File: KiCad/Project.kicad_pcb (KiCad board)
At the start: 2 copper layers, 138.4 x 74.9 mm, 73 parts, among them IC1 ATMEGA328-P, IC2 ATTINY85-P, IC3 ATTINY85-P, M1 Motor, M2 Motor, P1 CONN_02X03, P2 CONN_01X02, P3 CONN_01X02, P4 CONN_01X02, P5 CONN_02X04, P6 CONN_02X03, P7 CONN_01X02, Q1 Q_NPN_BCE, Q2 Q_NPN_BCE, Q4 Q_NPN_BCE, Q5 NPN, SW4 SW_PUSH, U1 BlueSmirf, U2 LM317, U3 LM317, U6 SN754410NE, Y1 Crystal

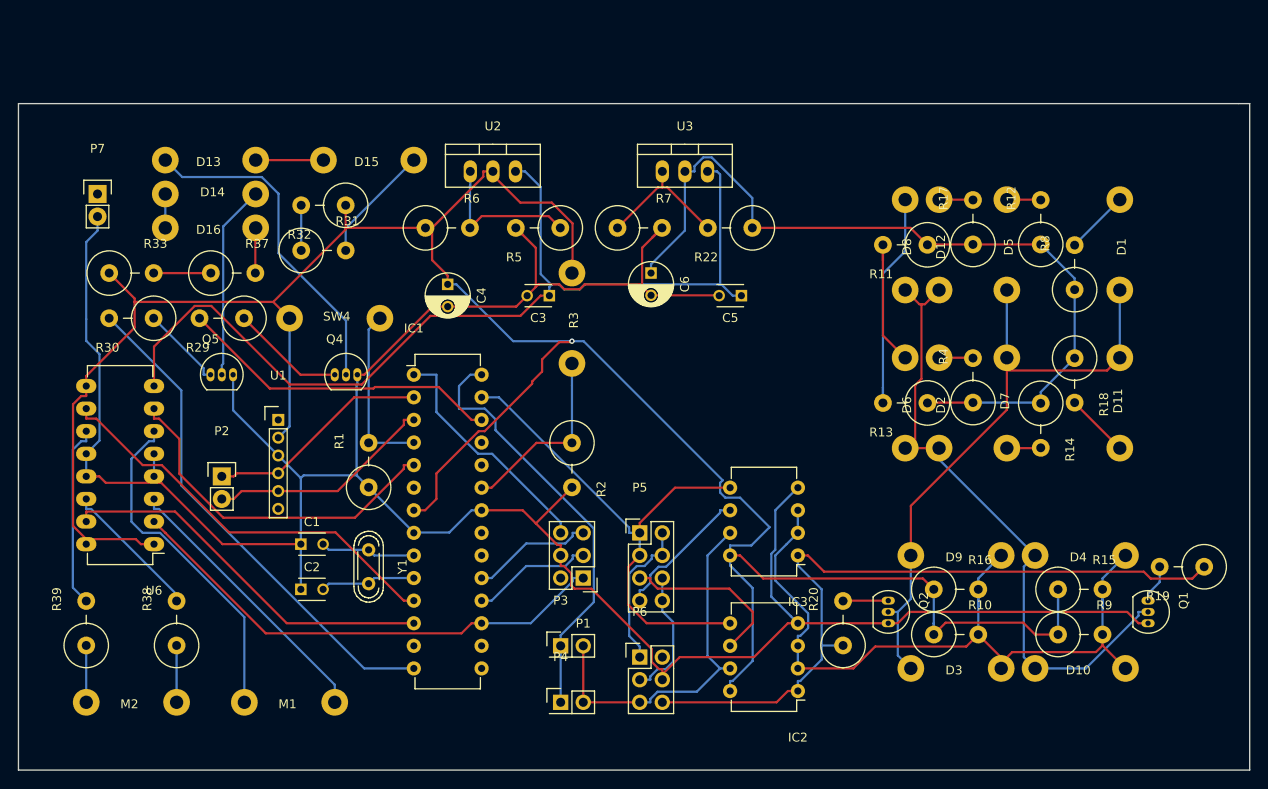
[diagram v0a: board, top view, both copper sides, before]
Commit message: Added smaller footprints
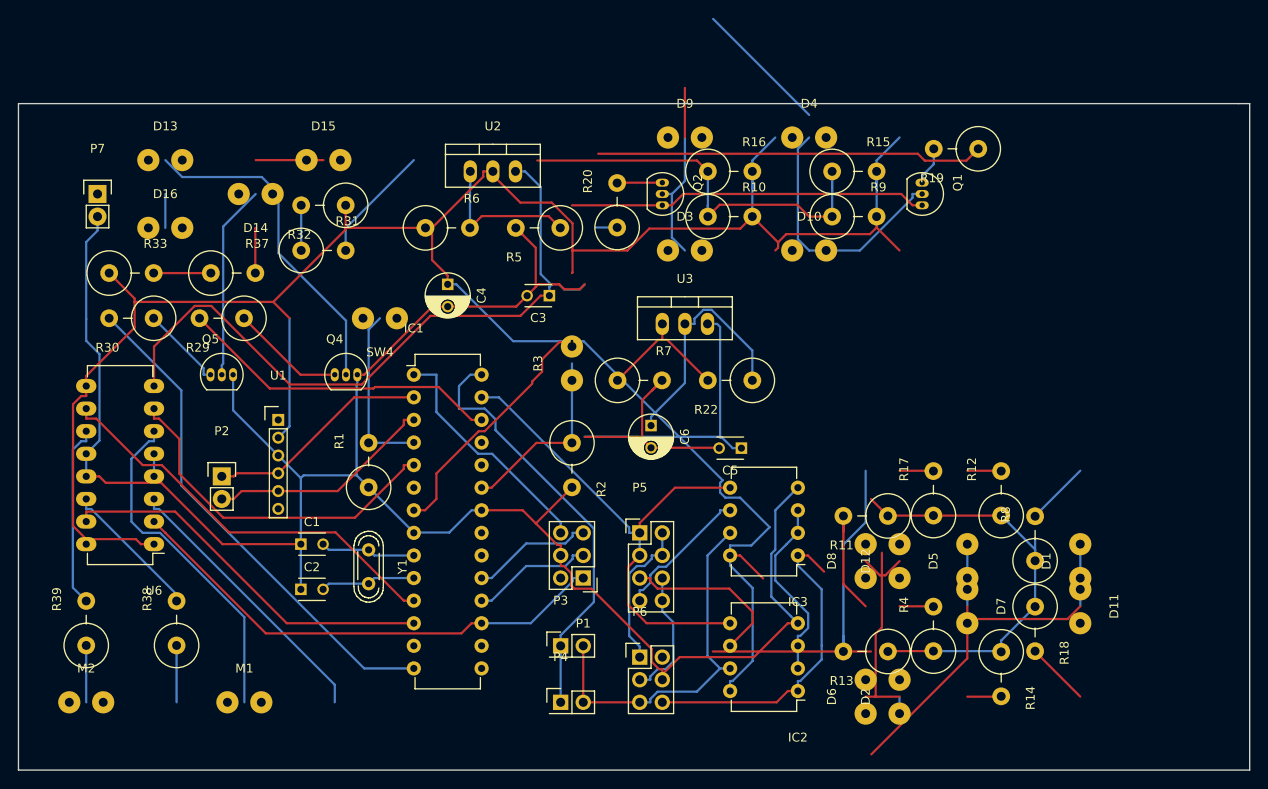
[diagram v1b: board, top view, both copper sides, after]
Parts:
- D1, D10, D11, D12, D13, D14, D15, D16, D2, D3, D4, D5, D6, D7, D8, D9, M1, M2, R3, SW4: footprint Wire_Connections_Bridges:WireConnection_1.50mmDrill -> Wire_Pads:SolderWirePad_2x_1mmDrill
- moved R15 53.4 mm to (152.4, 62.2)
- moved R16 53.4 mm to (138.4, 62.2)
- moved D10 53.4 mm to (147.3, 71.1)
- moved D3 53.4 mm to (133.3, 71.1)
- moved D4 53.4 mm to (147.3, 58.4)
- moved D9 53.4 mm to (133.3, 58.4)
- moved Q2 53.4 mm to (130.8, 63.5)
- moved R10 53.4 mm to (138.4, 67.3)
- moved R20 53.4 mm to (125.7, 66.0)
- moved R9 53.4 mm to (152.4, 67.3)
- moved R19 53.4 mm to (163.8, 59.7)
- moved Q1 53.4 mm to (160.0, 63.5)
- moved D12 30.8 mm to (157.5, 106.0)
- moved D8 30.8 mm to (153.7, 106.0)
- moved R11 30.8 mm to (153.7, 101.0)
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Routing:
- net (no net): track 0.00 -> 84.8 mm
- net Net-(IC1-Pad23): track 21.2 -> 88.1 mm, vias 0 -> 1
- net /IR/5V: track 290.0 -> 223.2 mm, vias 1 -> 0
- net Net-(D10-Pad1): track 71.3 -> 30.6 mm
- net Net-(D8-Pad2): track 25.6 -> 3.48 mm
- net Net-(D14-Pad1): track 21.9 -> 42.9 mm
- net Net-(D13-Pad1): track 37.8 -> 16.8 mm
- net /IR/3V: track 93.9 -> 76.1 mm
- net Net-(D6-Pad2): track 15.5 -> 28.3 mm
- net Net-(D13-Pad2): track 7.62 -> 0.00 mm
- net Net-(D1-Pad1): track 70.2 -> 64.6 mm
- net Net-(D14-Pad2): track 3.81 -> 0.00 mm
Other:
- net class Test added: clearance 0.2, trace_width 1, via_dia 1, via_drill 0.8

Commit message: Revert "Added smaller footprints"
This reverts commit 0613a684753a289cb87120d105616d3a60c555f9.
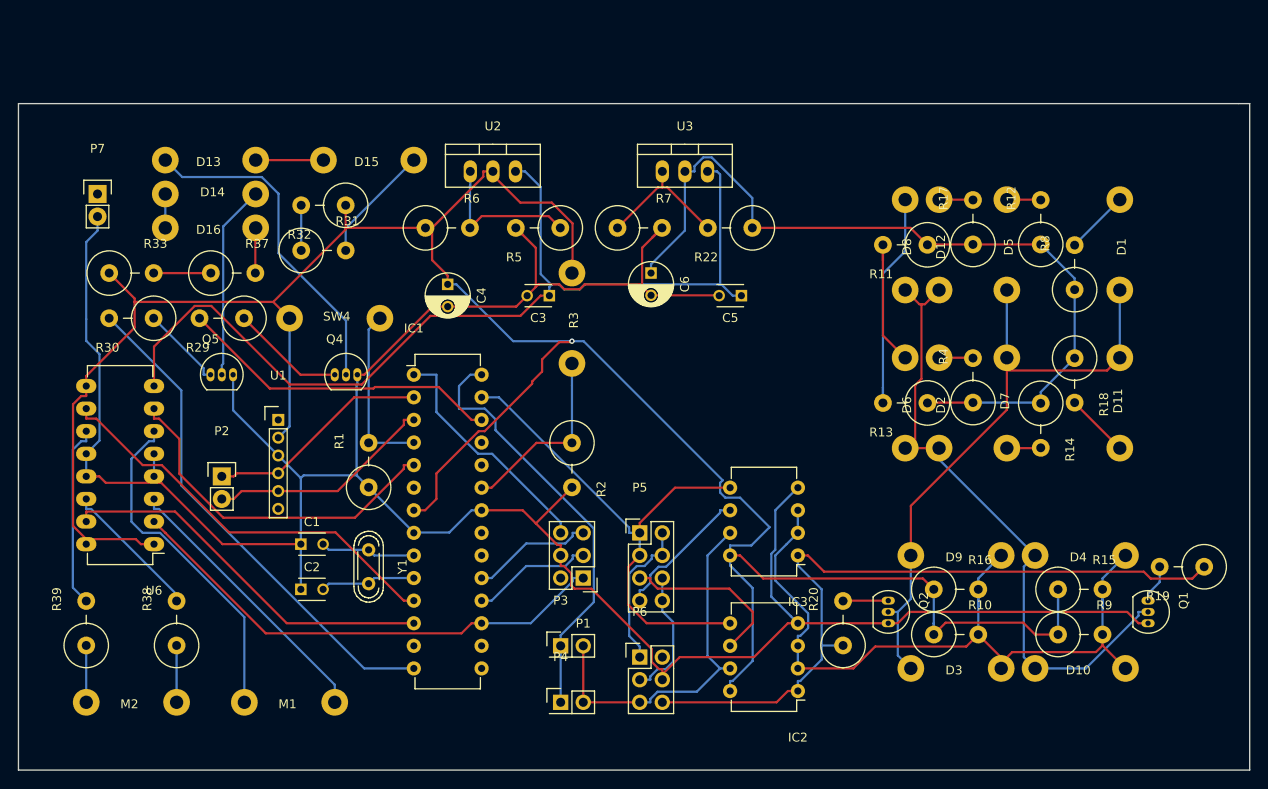
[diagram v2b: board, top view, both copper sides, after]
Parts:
- D1, D10, D11, D12, D13, D14, D15, D16, D2, D3, D4, D5, D6, D7, D8, D9, M1, M2, R3, SW4: footprint Wire_Pads:SolderWirePad_2x_1mmDrill -> Wire_Connections_Bridges:WireConnection_1.50mmDrill
- moved R15 53.4 mm to (177.8, 109.2)
- moved R16 53.4 mm to (163.8, 109.2)
- moved D10 53.4 mm to (172.7, 118.1)
- moved D3 53.4 mm to (158.8, 118.1)
- moved D4 53.4 mm to (172.7, 105.4)
- moved D9 53.4 mm to (158.8, 105.4)
- moved Q2 53.4 mm to (156.2, 110.5)
- moved R10 53.4 mm to (163.8, 114.3)
- moved R20 53.4 mm to (151.1, 113.0)
- moved R9 53.4 mm to (177.8, 114.3)
- moved R19 53.4 mm to (189.2, 106.7)
- moved Q1 53.4 mm to (185.4, 110.5)
- moved D12 30.8 mm to (161.9, 75.6)
- moved D8 30.8 mm to (158.1, 75.6)
- moved R11 30.8 mm to (158.1, 70.5)
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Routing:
- net (no net): track 84.8 -> 0.00 mm
- net Net-(IC1-Pad23): track 88.1 -> 21.2 mm, vias 1 -> 0
- net /IR/5V: track 223.2 -> 290.0 mm, vias 0 -> 1
- net Net-(D10-Pad1): track 30.6 -> 71.3 mm
- net Net-(D8-Pad2): track 3.48 -> 25.6 mm
- net Net-(D14-Pad1): track 42.9 -> 21.9 mm
- net Net-(D13-Pad1): track 16.8 -> 37.8 mm
- net /IR/3V: track 76.1 -> 93.9 mm
- net Net-(D6-Pad2): track 28.3 -> 15.5 mm
- net Net-(D13-Pad2): track 0.00 -> 7.62 mm
- net Net-(D1-Pad1): track 64.6 -> 70.2 mm
- net Net-(D14-Pad2): track 0.00 -> 3.81 mm
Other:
- net class Test removed
